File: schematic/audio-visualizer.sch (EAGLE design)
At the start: 18 parts, among them J3 455-1750-1-ND, U1 MSGEQ7P, U2 SN74AHCT125N

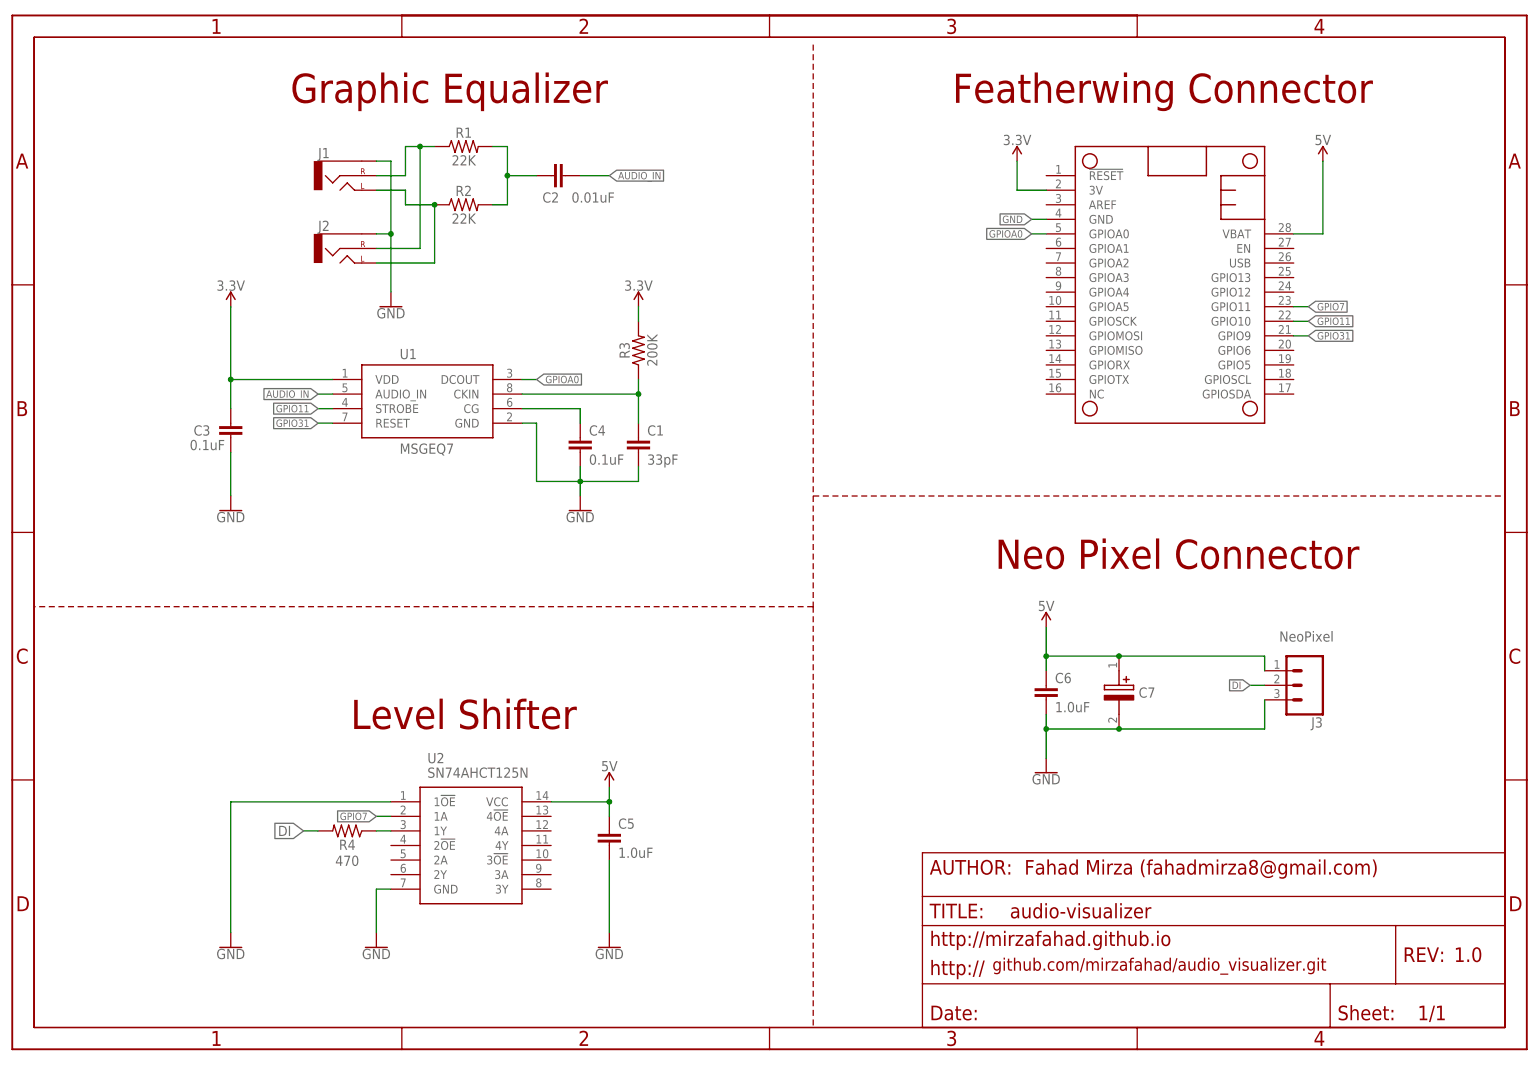
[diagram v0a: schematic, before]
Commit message: Updated folder structures.
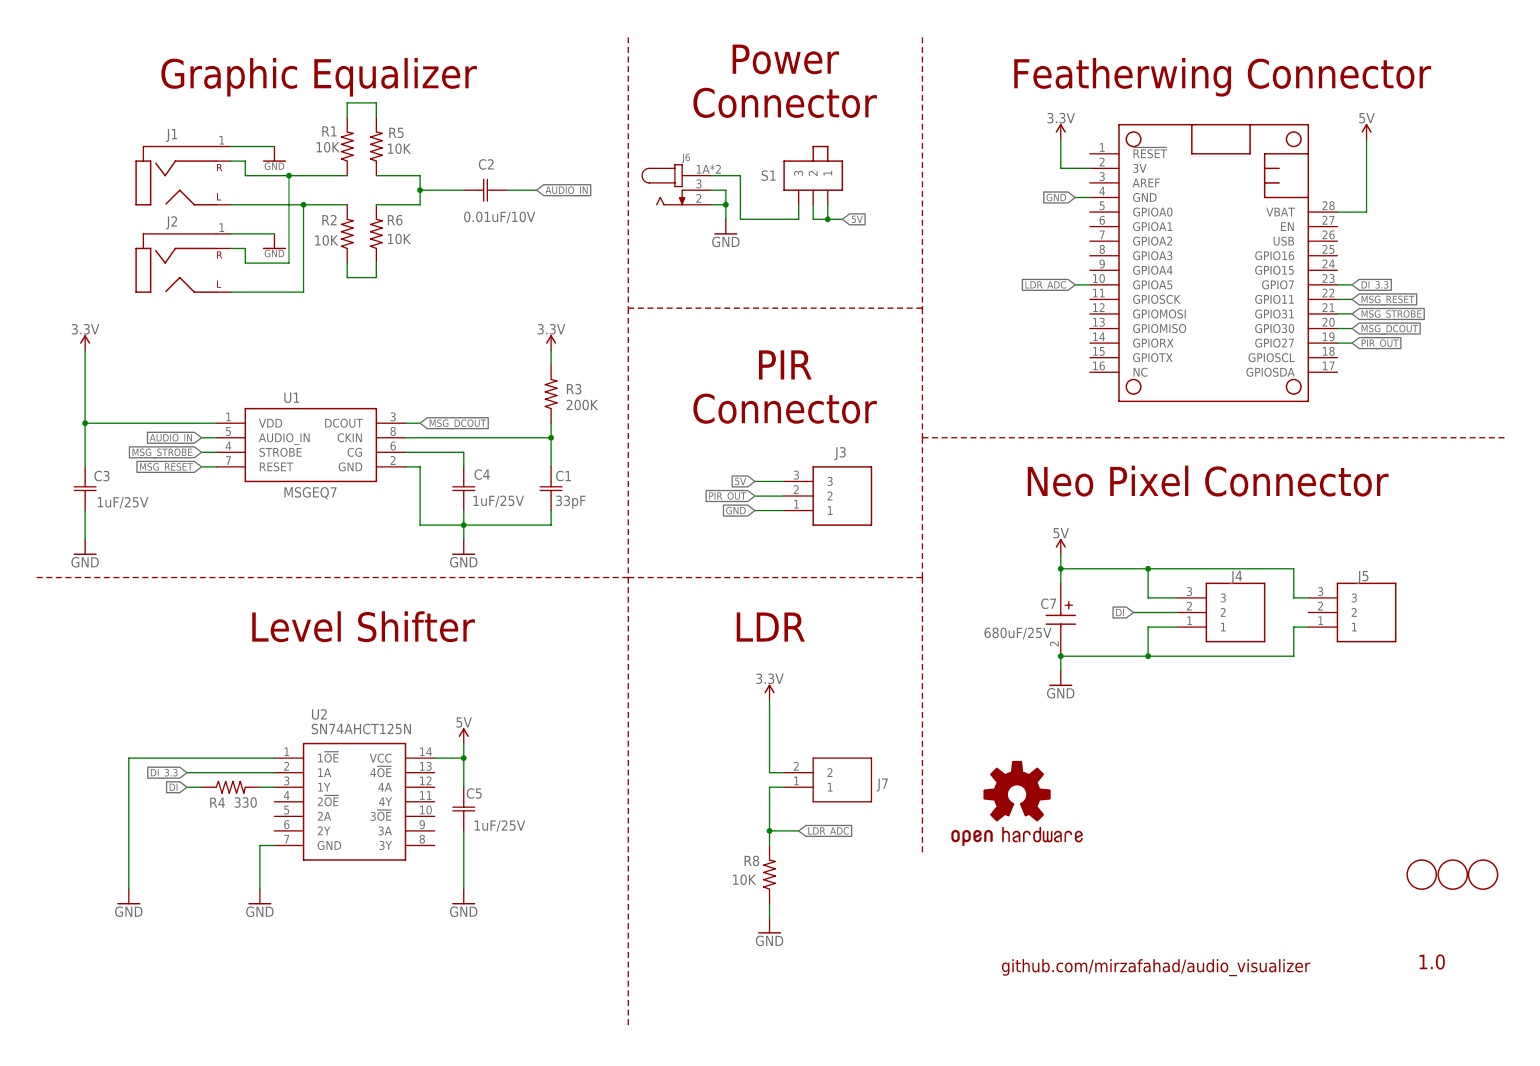
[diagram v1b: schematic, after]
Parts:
- removed C6: 1.0uF, SparkFun-Capacitors:1.0UF-0805-25V-(+80/-20%)
- removed PAGE1: FRAME_DINA4_L, dp_devices:FRAME_DINA4_L
- added J4, J5: 0022057035, SamacSys_Parts:0022057035
- added J6: PJ-002AH-SMT-TR, PersonalCollection:PJ-002AH-SMT-TR
- added J7: 22-05-7025, 22-05-7025:22-05-7025
- added LOGO1: OSHW-LOGOL-COPPER, SparkFun-Aesthetics:OSHW-LOGOL-COPPER
- added R5, R6, R8: 10K, SamacSys_Parts:R-US_R0805
- added S1: JS102011SAQN, JS102011SAQN:JS102011SAQN
- added U$2, U$3, U$4: FIDUCIAL, adafruit:FIDUCIAL
- C1: device SparkFun-Capacitors:1.0UF-0805-25V-(+80/-20%) -> SamacSys_Parts:CAP_0805
- C2: value 0.01uF -> 0.01uF/10V; device SparkFun-Capacitors:1.0UF-0805-25V-(+80/-20%) -> SamacSys_Parts:CAP_0805
- C3, C4: value 0.1uF -> 1uF/25V; device SparkFun-Capacitors:1.0UF-0805-25V-(+80/-20%) -> SamacSys_Parts:CAP_0805
- C5: value 1.0uF -> 1uF/25V; device SparkFun-Capacitors:1.0UF-0805-25V-(+80/-20%) -> SamacSys_Parts:CAP_0805
- C7: value 10TLV1000M10X10.5 -> 680uF/25V; device 10TLV1000M10X10.5:10TLV1000M10X10.5 -> SamacSys_Parts:EEE-FK1A681P
- J1, J2: value (none) -> SJ-3523-SMT-TR; device SparkFun-Connectors:AUDIO_JACK_2.5MM_HOLESONLY -> SamacSys_Parts:SJ-3523-SMT-TR
- J3: value 455-1750-1-ND -> 0022057035; device SparkFun-Connectors:CONN_03 -> SamacSys_Parts:0022057035
- MS1: value FEATHERWING_NODIM -> FEATHERWING_JUST_PINS; device adafruit:FEATHERWING_NODIM -> adafruit:FEATHERWING_JUST_PINS
- R1, R2: value 22K -> 10K; device SparkFun-Resistors:RESISTOR0805 -> SamacSys_Parts:R-US_R0805
- R3: device SparkFun-Resistors:RESISTOR0805 -> PersonalCollection:R-US_R0805
- R4: value 470 -> 330; device SparkFun-Resistors:RESISTOR0805 -> SamacSys_Parts:R-US_R0805
- U1: device SparkFun-IC-Special-Function:MSGEQ7DIL -> SamacSys_Parts:MSGEQ7DIL
- U2: device SN74AHCT125N:SN74AHCT125N -> SamacSys_Parts:SN74AHCT125N
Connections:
- removed net GPIO11: MS1.GPIO10, U1.STROBE
- removed net GPIO31: MS1.GPIO9, U1.RESET
- removed net GPIO7: MS1.GPIO11, U2.1A
- removed net GPIOA0: MS1.GPIOA0, U1.DCOUT
- new net DI_3.3: MS1.GPIO7, U2.1A
- new net LDR_ADC: J7.1, MS1.GPIOA5, R8.2
- new net MSG_DCOUT: MS1.GPIO30, U1.DCOUT
- new net MSG_RESET: MS1.GPIO11, U1.RESET
- new net MSG_STROBE: MS1.GPIO31, U1.STROBE
- new net N$10: J6.1, S1.3
- new net N$4: U2.1!OE
- new net N$7: J1.5, J2.5, R2.2
- new net N$9: J1.2, J2.2, R1.1
- new net PIR_OUT: J3.2, MS1.GPIO27
- net 3.3V: now also J7.2
- net 5V: now also J3.3, J4.3, J5.3, S1.1, S1.2; no longer C6.1, J3.1
- net DI: now also J4.2, R4.1; no longer J3.2, R4.2
- net GND: now also J1.1, J2.1, J3.1, J4.1, J5.1, J6.2, J6.3, R8.1; no longer C6.2, J1.SLEEVE, J2.SLEEVE, J3.3, U2.1!OE
- net N$1: now also R1.2, R5.2; no longer J1.RIGHT, J2.RIGHT, R1.1
- net N$2: now also R6.1; no longer J1.LEFT, J2.LEFT
- net N$3: now also R5.1, R6.2; no longer R1.2, R2.2
- net N$8: now also R4.2; no longer R4.1
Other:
- note added: "LDR"
- note added: "PIR Connector"
- note added: "Power Connector"
- note added: "github.com/mirzafahad/audio_visualizer"
- note removed: "NeoPixel"
- note removed: "github.com/mirzafahad/audio_visualizer.git"
- moved on the sheet: R1, R2, R3, R4, U1, U2
